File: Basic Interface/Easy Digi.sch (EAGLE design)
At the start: 5 parts

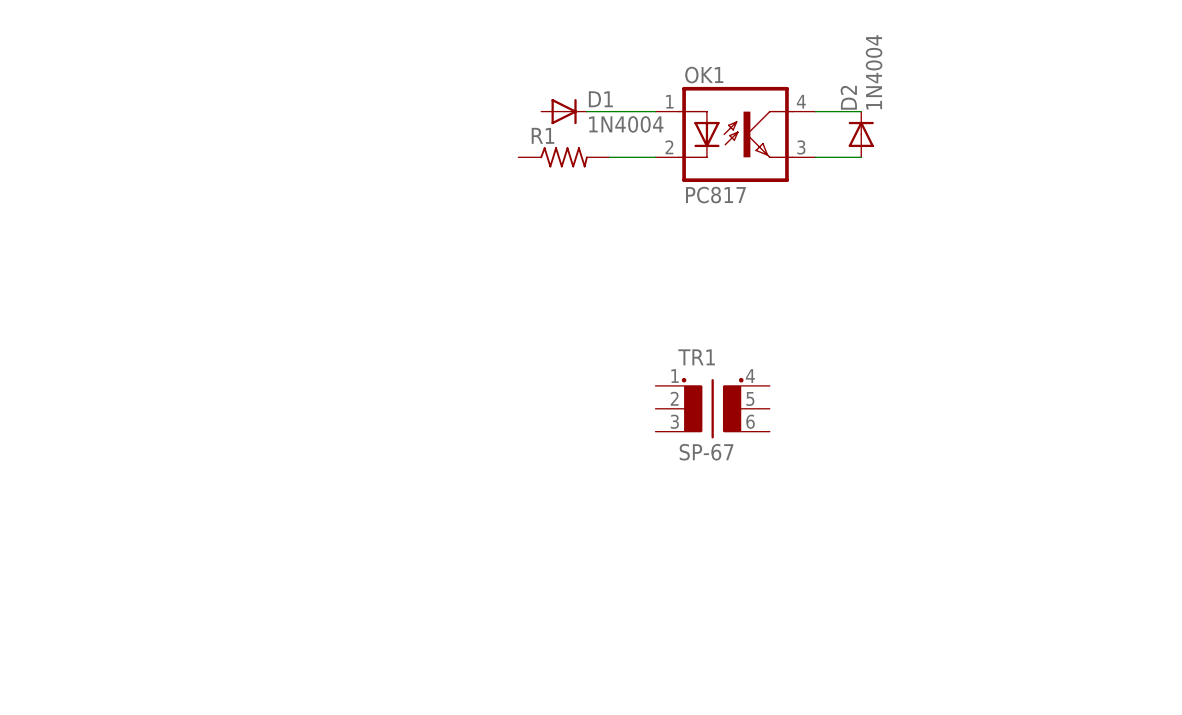
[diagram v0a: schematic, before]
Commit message: Easy Digi Updates
Note schematic of Easy Digi Board
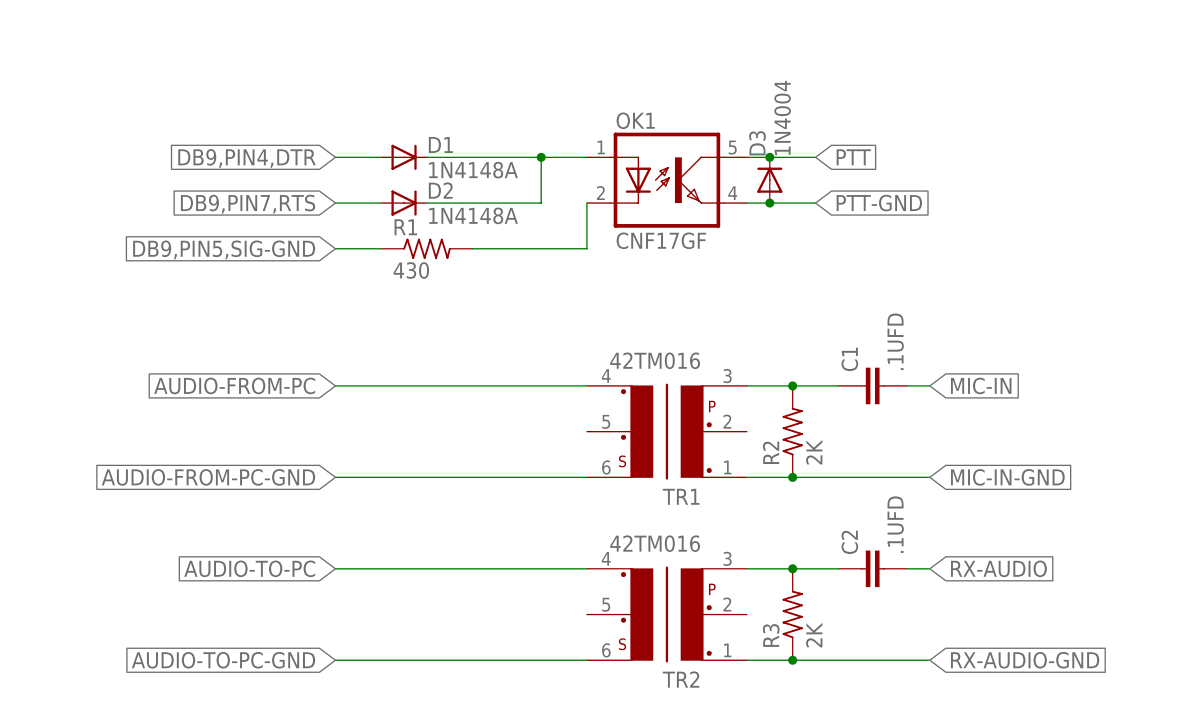
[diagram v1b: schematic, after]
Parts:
- added C1, C2: .1UFD, capacitor-wima:C5/3.5
- added D3: 1N4004, diode:1N4004
- added R2, R3: 2K, resistor:R-US_0204/7
- added TR2: 42TM016, trafo-xicon:42TM016
- D1, D2: value 1N4004 -> 1N4148A; device diode:1N4004 -> diode:1N4148DO35-10
- OK1: value PC817 -> CNF17GF; device optocoupler:PC817 -> optocoupler:CNF17GF
- R1: value (none) -> 430
- TR1: value SP-67 -> 42TM016; device trafo:SP-67 -> trafo-xicon:42TM016
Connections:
- removed net N$2 (its old number): D2.C, OK1.COL
- removed net N$4: D1.C, OK1.A
- new net AUDIO-FROM-PC: TR1.4
- new net AUDIO-FROM-PC-GND: TR1.6
- new net AUDIO-TO-PC: TR2.4
- new net AUDIO-TO-PC-GND: TR2.6
- new net DB9,PIN4,DTR: D1.A
- new net DB9,PIN5,SIG-GND: R1.1
- new net DB9,PIN7,RTS: D2.A
- new net MIC-IN: C1.2
- new net MIC-IN-GND: R2.1, TR1.1
- new net N$5: C1.1, R2.2, TR1.3
- new net N$7: C2.1, R3.2, TR2.3
- new net PTT: D3.C, OK1.COL
- new net PTT-GND: D3.A, OK1.EMIT
- new net RX-AUDIO: C2.2
- new net RX-AUDIO-GND: R3.1, TR2.1
- net N$1: now also D1.C, D2.C, OK1.A; no longer D2.A, OK1.EMIT
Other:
- moved on the sheet: OK1, R1
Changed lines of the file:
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@@
 <?xml version="1.0" encoding="utf-8"?>
 <!DOCTYPE eagle SYSTEM "eagle.dtd">
-<eagle version="7.1.0">
+<eagle version="6.5.0">
 <drawing>
 <settings>
@@
 </classes>
 <parts>
-<part name="TR1" library="trafo" deviceset="SP-67" device=""/>
-<part name="D1" library="diode" deviceset="1N4004" device=""/>
-<part name="D2" library="diode" deviceset="1N4004" device=""/>
-<part name="R1" library="resistor" deviceset="R-US_" device="0204/7"/>
-<part name="OK1" library="optocoupler" deviceset="PC817" device=""/>
+<part name="D1" library="diode" deviceset="1N4148" device="DO35-10" value="1N4148A"/>
+<part name="D2" library="diode" deviceset="1N4148" device="DO35-10" value="1N4148A"/>
+<part name="OK1" library="optocoupler" deviceset="CNF17GF" device=""/>
+<part name="D3" library="diode" deviceset="1N4004" device=""/>
+<part name="R1" library="resistor" deviceset="R-US_" device="0204/7" value="430"/>
+<part name="R2" library="resistor" deviceset="R-US_" device="0204/7" value="2K"/>
+<part name="R3" library="resistor" deviceset="R-US_" device="0204/7" value="2K"/>
+<part name="TR1" library="trafo-xicon" deviceset="42T?*" device="M" technology="016"/>
+<part name="TR2" library="trafo-xicon" deviceset="42T?*" device="M" technology="016"/>
+<part name="C1" library="capacitor-wima" deviceset="C" device="5/3.5" value=".1UFD"/>
+<part name="C2" library="capacitor-wima" deviceset="C" device="5/3.5" value=".1UFD"/>
 </parts>
 <sheets>
@@
 </plain>
 <instances>
-<instance part="TR1" gate="G$1" x="71.12" y="17.78"/>
-<instance part="D1" gate="1" x="55.88" y="50.8"/>
-<instance part="D2" gate="1" x="88.9" y="48.26" rot="R90"/>
-<instance part="R1" gate="G$1" x="55.88" y="45.72"/>
-<instance part="OK1" gate="A" x="76.2" y="48.26"/>
+<instance part="D1" gate="G$1" x="38.1" y="45.72"/>
+<instance part="D2" gate="G$1" x="38.1" y="40.64"/>
+<instance part="OK1" gate="A" x="68.58" y="43.18"/>
+<instance part="D3" gate="1" x="78.74" y="43.18" rot="R90"/>
+<instance part="R1" gate="G$1" x="40.64" y="35.56"/>
+<instance part="R2" gate="G$1" x="81.28" y="15.24" rot="R90"/>
+<instance part="R3" gate="G$1" x="81.28" y="-5.08" rot="R90"/>
+<instance part="TR1" gate="G$1" x="68.58" y="15.24" rot="R180"/>
+<instance part="TR2" gate="G$1" x="68.58" y="-5.08" rot="R180"/>
+<instance part="C1" gate="G$1" x="88.9" y="20.32" rot="R90"/>
+<instance part="C2" gate="G$1" x="88.9" y="0" rot="R90"/>
 </instances>
 <busses>
@@
 <net name="N$1" class="0">
 <segment>
-<pinref part="D2" gate="1" pin="A"/>
-<wire x1="83.82" y1="45.72" x2="88.9" y2="45.72" width="0.1524" layer="91"/>
+<pinref part="D1" gate="G$1" pin="C"/>
+<pinref part="OK1" gate="A" pin="A"/>
+<wire x1="40.64" y1="45.72" x2="53.34" y2="45.72" width="0.1524" layer="91"/>
+<pinref part="D2" gate="G$1" pin="C"/>
+<wire x1="53.34" y1="45.72" x2="58.42" y2="45.72" width="0.1524" layer="91"/>
+<wire x1="40.64" y1="40.64" x2="53.34" y2="40.64" width="0.1524" layer="91"/>
+<wire x1="53.34" y1="40.64" x2="53.34" y2="45.72" width="0.1524" layer="91"/>
+<junction x="53.34" y="45.72"/>
+</segment>
+</net>
+<net name="N$2" class="0">
+<segment>
+<pinref part="R1" gate="G$1" pin="2"/>
+<wire x1="45.72" y1="35.56" x2="58.42" y2="35.56" width="0.1524" layer="91"/>
+<pinref part="OK1" gate="A" pin="C"/>
+<wire x1="58.42" y1="35.56" x2="58.42" y2="40.64" width="0.1524" layer="91"/>
+</segment>
+</net>
+<net name="PTT" class="0">
+<segment>
+<pinref part="OK1" gate="A" pin="COL"/>
+<pinref part="D3" gate="1" pin="C"/>
+<wire x1="76.2" y1="45.72" x2="78.74" y2="45.72" width="0.1524" layer="91"/>
+<wire x1="83.82" y1="45.72" x2="78.74" y2="45.72" width="0.1524" layer="91"/>
+<junction x="78.74" y="45.72"/>
+<label x="83.82" y="45.72" size="1.778" layer="95" xref="yes"/>
+</segment>
+</net>
+<net name="PTT-GND" class="0">
+<segment>
 <pinref part="OK1" gate="A" pin="EMIT"/>
-</segment>
-</net>
-<net name="N$2" class="0">
-<segment>
-<pinref part="D2" gate="1" pin="C"/>
-<wire x1="88.9" y1="50.8" x2="83.82" y2="50.8" width="0.1524" layer="91"/>
-<pinref part="OK1" gate="A" pin="COL"/>
-</segment>
-</net>
-<net name="N$3" class="0">
-<segment>
-<pinref part="R1" gate="G$1" pin="2"/>
-<wire x1="66.04" y1="45.72" x2="60.96" y2="45.72" width="0.1524" layer="91"/>
-<pinref part="OK1" gate="A" pin="C"/>
-</segment>
-</net>
-<net name="N$4" class="0">
-<segment>
-<pinref part="OK1" gate="A" pin="A"/>
-<pinref part="D1" gate="1" pin="C"/>
-<wire x1="66.04" y1="50.8" x2="58.42" y2="50.8" width="0.1524" layer="91"/>
-</segment>
-</net>
+<pinref part="D3" gate="1" pin="A"/>
+<wire x1="76.2" y1="40.64" x2="78.74" y2="40.64" width="0.1524" layer="91"/>
+<wire x1="83.82" y1="40.64" x2="78.74" y2="40.64" width="0.1524" layer="91"/>
+<junction x="78.74" y="40.64"/>
+<label x="83.82" y="40.64" size="1.778" layer="95" xref="yes"/>
+</segment>
+</net>
+<net name="N$5" class="0">
+<segment>
+<pinref part="TR1" gate="G$1" pin="3"/>
+<pinref part="R2" gate="G$1" pin="2"/>
+<wire x1="76.2" y1="20.32" x2="81.28" y2="20.32" width="0.1524" layer="91"/>
+<pinref part="C1" gate="G$1" pin="1"/>
+<wire x1="86.36" y1="20.32" x2="81.28" y2="20.32" width="0.1524" layer="91"/>
+<junction x="81.28" y="20.32"/>
+</segment>
+</net>
+<net name="MIC-IN-GND" class="0">
+<segment>
+<pinref part="R2" gate="G$1" pin="1"/>
+<pinref part="TR1" gate="G$1" pin="1"/>
+<wire x1="81.28" y1="10.16" x2="76.2" y2="10.16" width="0.1524" layer="91"/>
+<wire x1="96.52" y1="10.16" x2="81.28" y2="10.16" width="0.1524" layer="91"/>
+<junction x="81.28" y="10.16"/>
+<label x="96.52" y="10.16" size="1.778" layer="95" xref="yes"/>
+</segment>
+</net>
+<net name="N$7" class="0">
+<segment>
+<pinref part="C2" gate="G$1" pin="1"/>
+<pinref part="R3" gate="G$1" pin="2"/>
+<wire x1="86.36" y1="0" x2="81.28" y2="0" width="0.1524" layer="91"/>
+<pinref part="TR2" gate="G$1" pin="3"/>
+<wire x1="81.28" y1="0" x2="76.2" y2="0" width="0.1524" layer="91"/>
+<junction x="81.28" y="0"/>
+</segment>
+</net>
+<net name="RX-AUDIO-GND" class="0">
+<segment>
+<pinref part="R3" gate="G$1" pin="1"/>
+<pinref part="TR2" gate="G$1" pin="1"/>
+<wire x1="81.28" y1="-10.16" x2="76.2" y2="-10.16" width="0.1524" layer="91"/>
+<wire x1="96.52" y1="-10.16" x2="81.28" y2="-10.16" width="0.1524" layer="91"/>
+<junction x="81.28" y="-10.16"/>
+<label x="96.52" y="-10.16" size="1.778" layer="95" xref="yes"/>
+</segment>
+</net>
+<net name="AUDIO-FROM-PC" class="0">
+<segment>
+<pinref part="TR1" gate="G$1" pin="4"/>
+<wire x1="58.42" y1="20.32" x2="30.48" y2="20.32" width="0.1524" layer="91"/>
+<label x="30.48" y="20.32" size="1.778" layer="95" rot="R180" xref="yes"/>
+</segment>
+</net>
+<net name="AUDIO-FROM-PC-GND" class="0">
+<segment>
+<pinref part="TR1" gate="G$1" pin="6"/>
+<wire x1="58.42" y1="10.16" x2="30.48" y2="10.16" width="0.1524" layer="91"/>
+<label x="30.48" y="10.16" size="1.778" layer="95" rot="R180" xref="yes"/>
+</segment>
+</net>
+<net name="AUDIO-TO-PC" class="0">
+<segment>
+<pinref part="TR2" gate="G$1" pin="4"/>
+<wire x1="58.42" y1="0" x2="30.48" y2="0" width="0.1524" layer="91"/>
+<label x="30.48" y="0" size="1.778" layer="95" rot="R180" xref="yes"/>
+</segment>
+</net>
+<net name="AUDIO-TO-PC-GND" class="0">
+<segment>
+<pinref part="TR2" gate="G$1" pin="6"/>
+<wire x1="58.42" y1="-10.16" x2="30.48" y2="-10.16" width="0.1524" layer="91"/>
+<label x="30.48" y="-10.16" size="1.778" layer="95" rot="R180" xref="yes"/>
+</segment>
+</net>
+<net name="DB9,PIN4,DTR" class="0">
+<segment>
+<pinref part="D1" gate="G$1" pin="A"/>
+<wire x1="35.56" y1="45.72" x2="30.48" y2="45.72" width="0.1524" layer="91"/>
+<label x="30.48" y="45.72" size="1.778" layer="95" rot="R180" xref="yes"/>
+</segment>
+</net>
+<net name="DB9,PIN7,RTS" class="0">
+<segment>
+<pinref part="D2" gate="G$1" pin="A"/>
+<wire x1="35.56" y1="40.64" x2="30.48" y2="40.64" width="0.1524" layer="91"/>
+<label x="30.48" y="40.64" size="1.778" layer="95" rot="R180" xref="yes"/>
+</segment>
+</net>
+<net name="DB9,PIN5,SIG-GND" class="0">
+<segment>
+<pinref part="R1" gate="G$1" pin="1"/>
+<wire x1="35.56" y1="35.56" x2="30.48" y2="35.56" width="0.1524" layer="91"/>
+<label x="30.48" y="35.56" size="1.778" layer="95" rot="R180" xref="yes"/>
+</segment>
+</net>
+<net name="MIC-IN" class="0">
+<segment>
+<pinref part="C1" gate="G$1" pin="2"/>
+<wire x1="93.98" y1="20.32" x2="96.52" y2="20.32" width="0.1524" layer="91"/>
+<label x="96.52" y="20.32" size="1.778" layer="95" xref="yes"/>
+</segment>
+</net>
+<net name="RX-AUDIO" class="0">
+<segment>
+<pinref part="C2" gate="G$1" pin="2"/>
+<wire x1="93.98" y1="0" x2="96.52" y2="0" width="0.1524" layer="91"/>
+<label x="96.52" y="0" size="1.778" layer="95" xref="yes"/>
+</segment>
+</net>
